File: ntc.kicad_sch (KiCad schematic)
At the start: 4 parts, among them J10 Conn_01x02_Pin, J11 Conn_01x02_Pin, J12 Conn_01x02_Pin, J13 Conn_01x02_Pin

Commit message: Doing placement
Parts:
- J10, J11, J12, J13: footprint Connector_JST:JST_PH_S2B-PH-SM4-TB_1x02-1MP_P2.00mm_Horizontal -> Connector_JST:JST_GH_SM02B-GHS-TB_1x02-1MP_P1.25mm_Horizontal

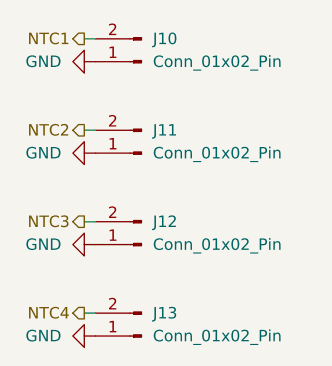
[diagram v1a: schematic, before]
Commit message: Pushing
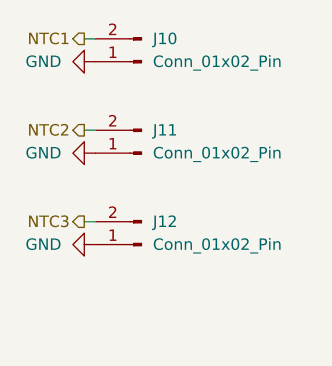
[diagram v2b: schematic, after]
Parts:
- removed J13: Conn_01x02_Pin, Connector_JST:JST_GH_SM02B-GHS-TB_1x02-1MP_P1.25mm_Horizontal, symbol Connector:Conn_01x02_Pin
